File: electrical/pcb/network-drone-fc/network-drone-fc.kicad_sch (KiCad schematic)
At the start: 78 parts, among them J1 U.FL-R-SMT-1, J2 TYPE-C 16PIN 2MD, J3 U.FL GPS, J4 ESC, J5 I2C port, J7 Charging board, U1 ESP32-S3FN8, U2 USBLC6-2SC6, U3 AP63205WU-7, U4 TLV75733PDBVR, U5 TPS7A2033PDBVR, U6 ICM-42688-P, U7 BMP581, U8 MAX-M10S, X1 Q22FA12800101

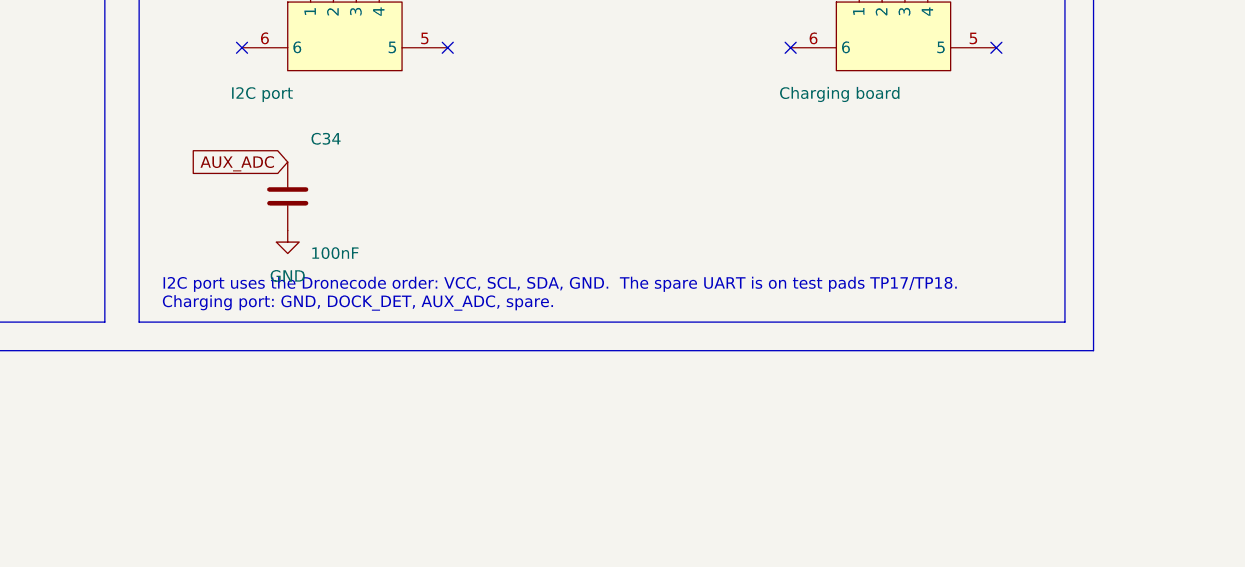
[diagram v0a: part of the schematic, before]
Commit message: Schematic: drop the spare-UART note from the connector sheet
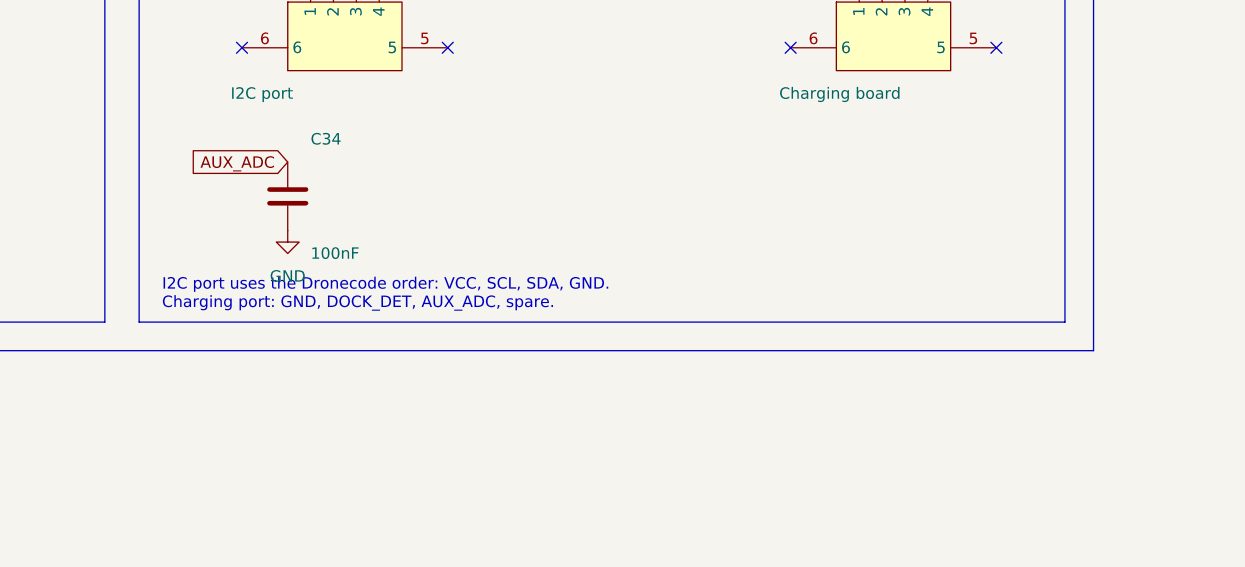
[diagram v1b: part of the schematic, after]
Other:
- note added: "I2C port uses the Dronecode order: VCC, SCL, SDA, GND. Charging port: GND, DOCK_DET, AUX_ADC, spare."
- note removed: "I2C port uses the Dronecode order: VCC, SCL, SDA, GND. The spare UART is on test pads TP17/TP18. Charging port: GND, DOCK_DET, AUX_ADC, spare."
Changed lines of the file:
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@@
 		)
 	)
-	(text "I2C port uses the Dronecode order: VCC, SCL, SDA, GND.  The spare UART is on test pads TP17/TP18.\nCharging port: GND, DOCK_DET, AUX_ADC, spare."
+	(text "I2C port uses the Dronecode order: VCC, SCL, SDA, GND.\nCharging port: GND, DOCK_DET, AUX_ADC, spare."
 		(exclude_from_sim no)
 		(at 304.8 248.92 0)
